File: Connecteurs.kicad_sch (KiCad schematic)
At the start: 22 parts, among them J10 Conn_01x02_Pin, J11 Conn_01x02_Pin, J2 USB_C_Receptacle_PowerOnly_6P, J3 Conn_02x07_Odd_Even, Q7 AO3401A

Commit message: t
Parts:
- BT1: footprint (none) -> Composants_Perso:BH-18650-4
- J2: footprint Composants_Perso:Connector_GT-USB-7002A -> Composants_Perso:UC18-0B06F68011; LCSC (none) -> C963365
- J3: LCSC (none) -> C42462827
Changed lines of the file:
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@@
 			)
 		)
-		(property "LCSC" ""
+		(property "LCSC" "C42462827"
 			(at 219.71 44.45 0)
 			(effects
@@
 			)
 		)
-		(property "Footprint" "Composants_Perso:Connector_GT-USB-7002A"
+		(property "Footprint" "Composants_Perso:UC18-0B06F68011"
 			(at 60.96 41.91 0)
 			(effects
@@
 			)
 		)
-		(property "LCSC" ""
+		(property "LCSC" "C963365"
 			(at 57.15 44.45 0)
 			(effects
@@
 			)
 		)
-		(property "Footprint" ""
+		(property "Footprint" "Composants_Perso:BH-18650-4"
 			(at 106.68 106.426 90)
 			(effects

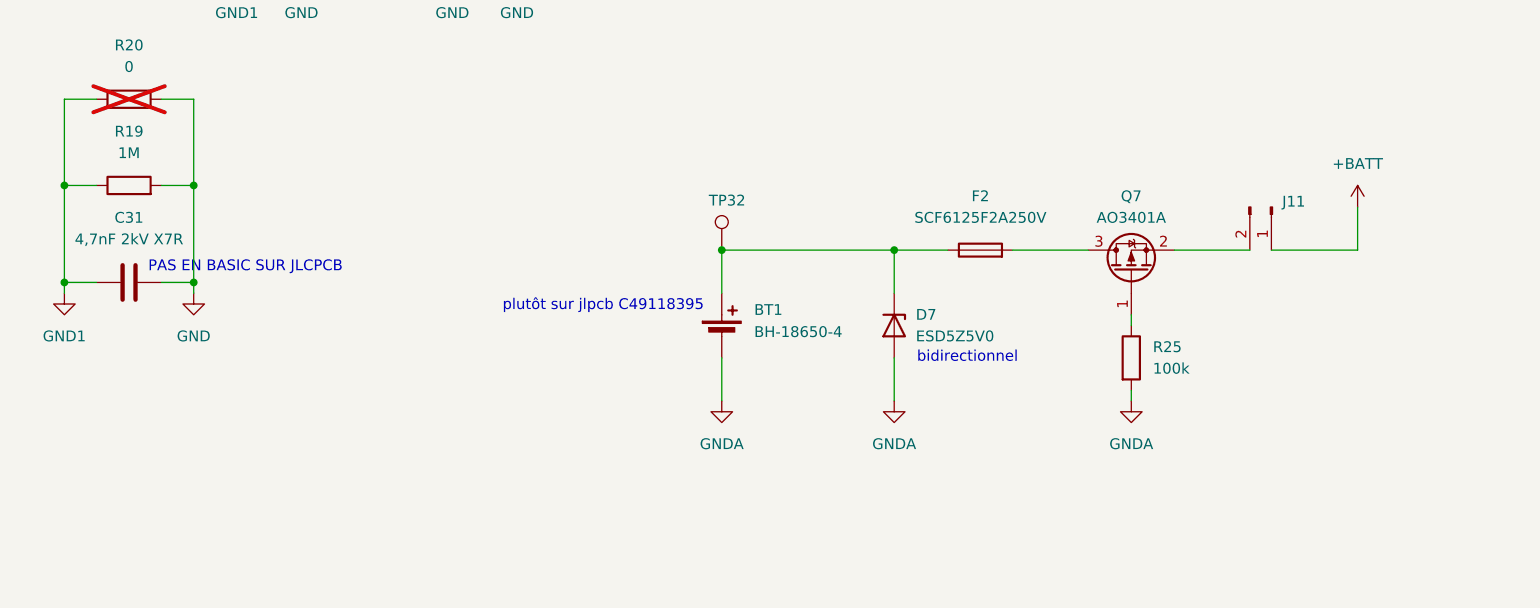
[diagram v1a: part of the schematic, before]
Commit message: t
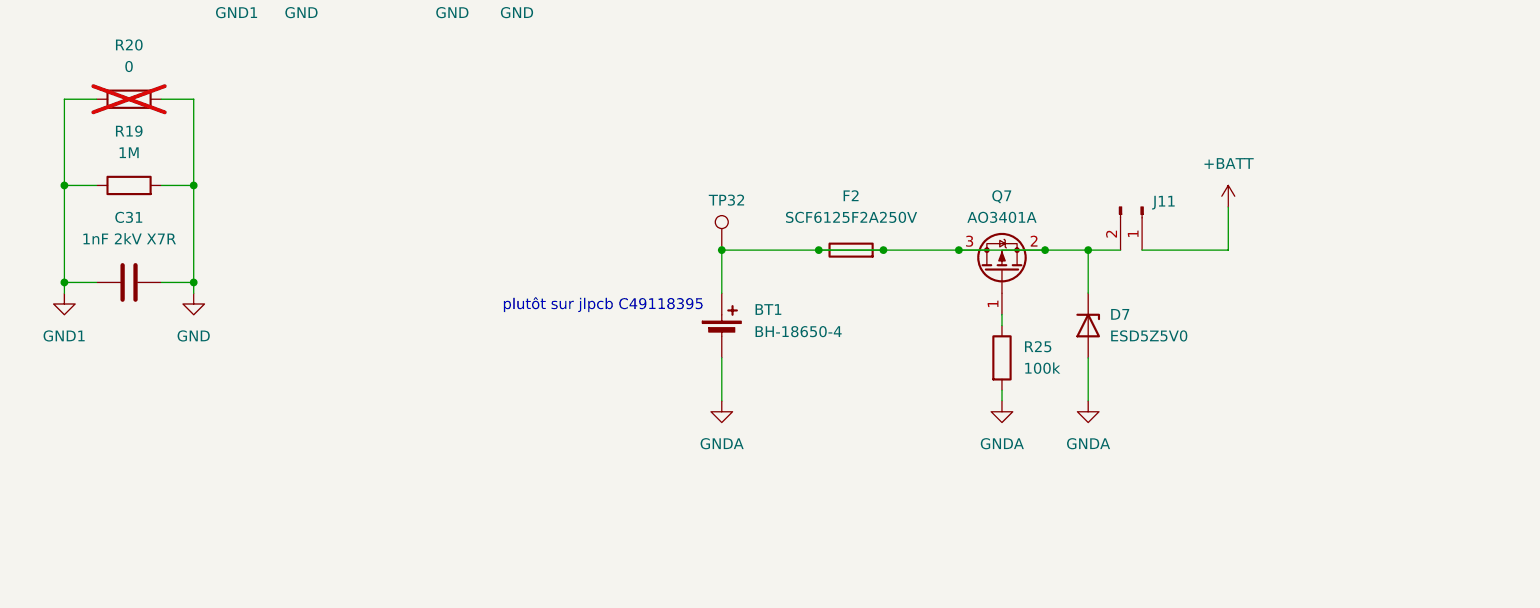
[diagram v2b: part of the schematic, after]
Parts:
- C31: value 4,7nF 2kV X7R -> 1nF 2kV X7R; footprint (none) -> Capacitor_SMD:C_1206_3216Metric; LCSC (none) -> C9196
- F1, F2: footprint (none) -> Composants_Perso:SCF6125F2A250V
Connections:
- net at J11.2 (Pin_2), Q7.2 (S): now also BT1.1 (+), D7.1 (K), F2.1, F2.2, Q7.3 (D), TP32.1
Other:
- note removed: "PAS EN BASIC SUR JLCPCB"
- note removed: "bidirectionnel"
- moved on the sheet: D7, F2, J11, Q7, R25
